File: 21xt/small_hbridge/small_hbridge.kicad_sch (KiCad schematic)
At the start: 3 parts, among them J1 Conn_01x03, J2 Conn_01x02, J3 Barrel_Jack

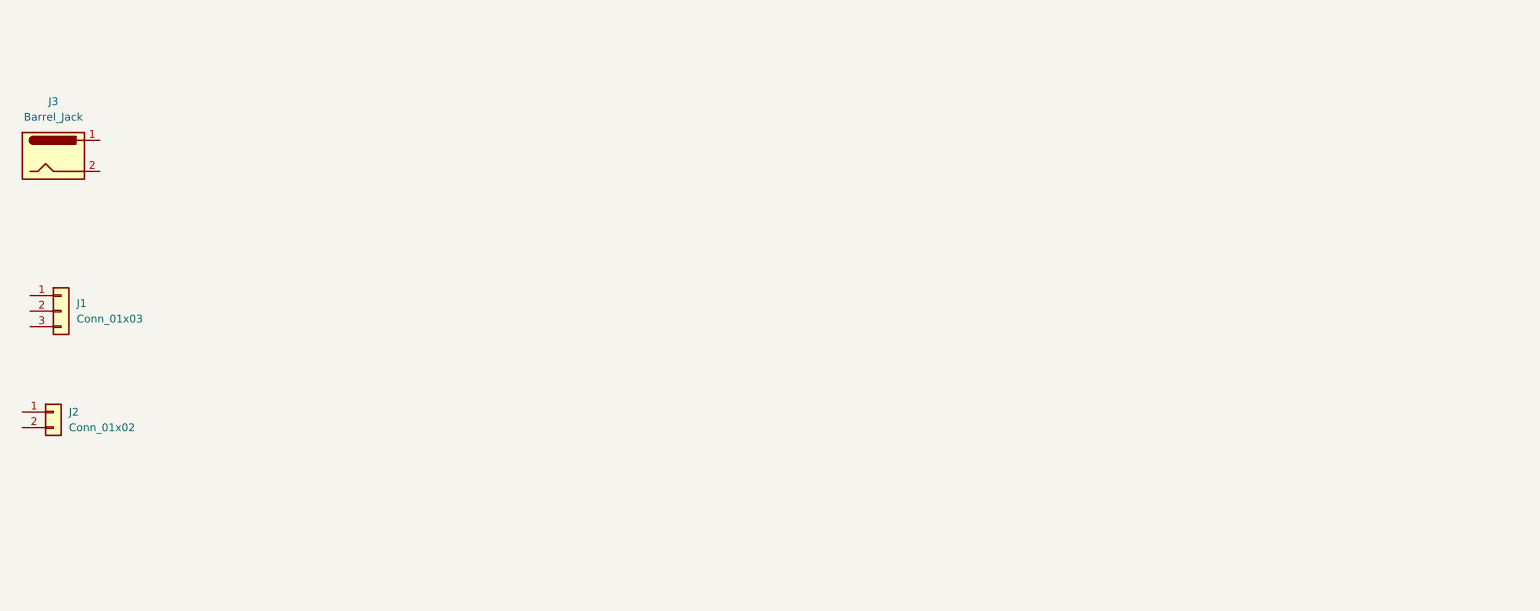
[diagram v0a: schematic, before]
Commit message: aaaaa
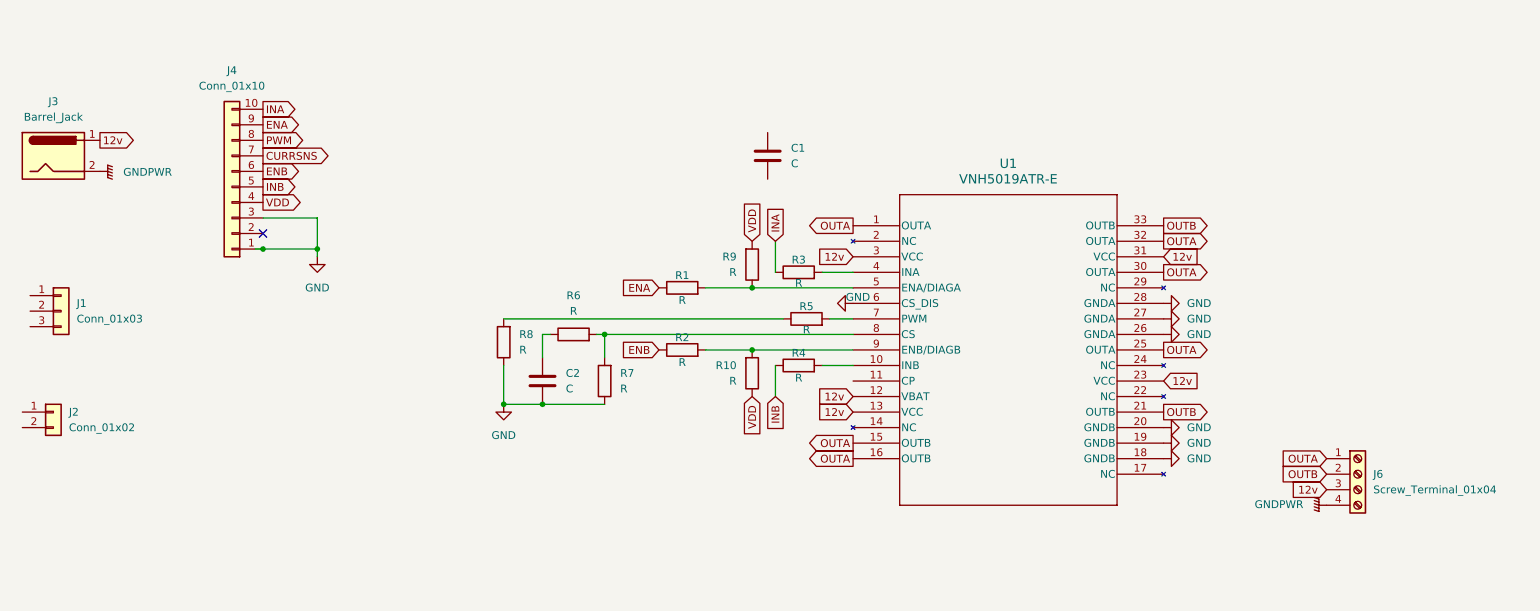
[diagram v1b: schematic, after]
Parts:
- added C1, C2: C, symbol Device:C
- added J4: Conn_01x10, symbol Connector_Generic:Conn_01x10
- added J6: Screw_Terminal_01x04, symbol Connector:Screw_Terminal_01x04
- added R1, R10, R2, R3, R4, R5, R6, R7, R8, R9: R, symbol Device:R
- added U1: VNH5019ATR-E, MultiPowerSO-30_STM, symbol dyno_inst_sym:VNH5019ATR-E
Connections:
- net 12v: now reaches J3.1
- net 12v: now also J6.3 (Pin_3), U1.12 (VBAT), U1.13 (VCC), U1.23 (VCC), U1.3 (VCC), U1.31 (VCC)
- net GNDPWR: now reaches J3.2
- net GNDPWR: now also J6.4 (Pin_4)
- new net: R5.1, R8.2
- new net: R5.2, U1.7 (PWM)
- new net: C2.1, R6.1
- new net: R3.2, U1.4 (INA)
- new net: R6.2, R7.2, U1.8 (CS)
- new net: R4.2, U1.10 (INB)
- new net: R1.2, R9.1, U1.5 (ENA/DIAGA)
- new net: R10.2, R2.2, U1.9 (ENB/DIAGB)
- new net CURRSNS: J4.7 (Pin_7)
- new net ENA: J4.9 (Pin_9), R1.1
- new net ENB: J4.6 (Pin_6), R2.1
- new net GND: C2.2, J4.1 (Pin_1), J4.3 (Pin_3), R7.1, R8.1, U1.18 (GNDB), U1.19 (GNDB), U1.20 (GNDB), U1.26 (GNDA), U1.27 (GNDA), U1.28 (GNDA), U1.6 (CS_DIS)
- new net INA: J4.10 (Pin_10), R3.1
- new net INB: J4.5 (Pin_5), R4.1
- new net OUTA: J6.1 (Pin_1), U1.1 (OUTA), U1.15 (OUTB), U1.16 (OUTB), U1.25 (OUTA), U1.30 (OUTA), U1.32 (OUTA)
- new net OUTB: J6.2 (Pin_2), U1.21 (OUTB), U1.33 (OUTB)
- new net PWM: J4.8 (Pin_8)
- new net VDD: J4.4 (Pin_4), R10.1, R9.2
- no-connect marks 0 -> 1

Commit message: ssss
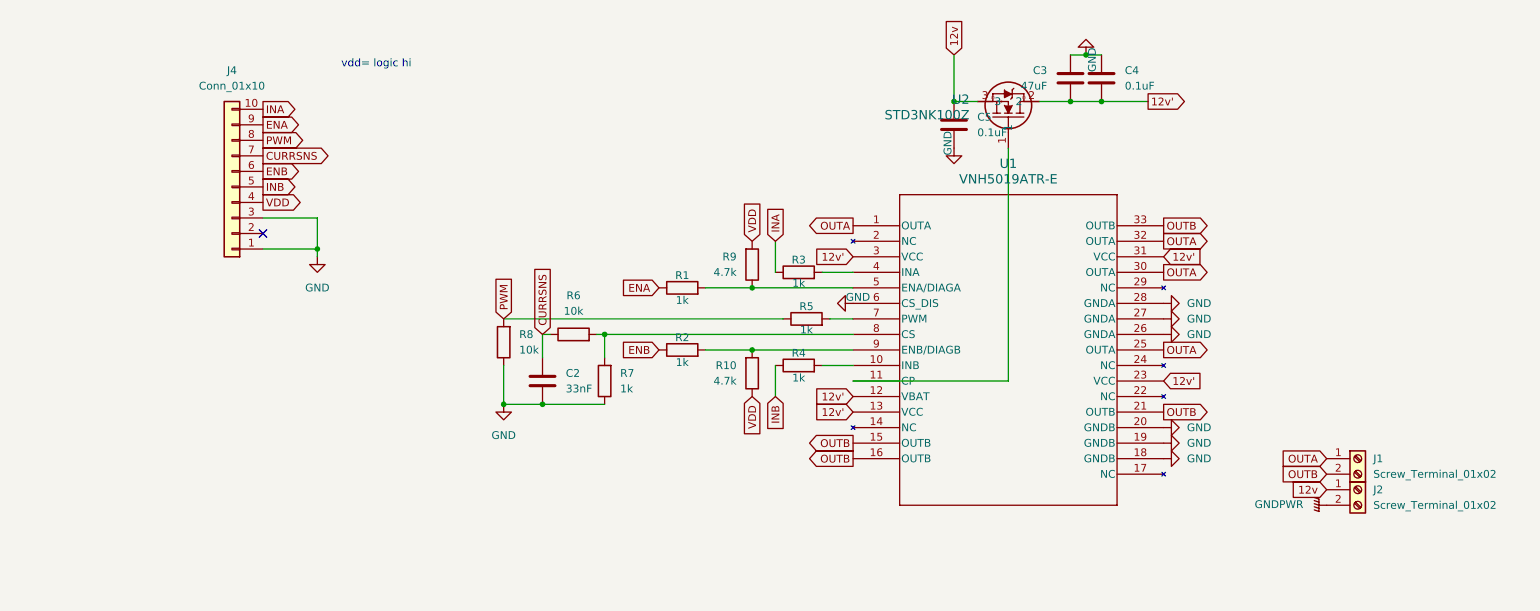
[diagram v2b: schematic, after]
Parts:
- removed C1: C, symbol Device:C
- removed J1: Conn_01x03, symbol Connector_Generic:Conn_01x03
- removed J2: Conn_01x02, symbol Connector_Generic:Conn_01x02
- removed J3: Barrel_Jack, symbol Connector:Barrel_Jack
- removed J6: Screw_Terminal_01x04, symbol Connector:Screw_Terminal_01x04
- added C3: 47uF, Capacitor_SMD:C_0603_1608Metric, symbol Device:C
- added C4, C5: 0.1uF, Capacitor_SMD:C_0603_1608Metric, symbol Device:C
- added J1, J2: Screw_Terminal_01x02, dynoinst_fp:CONN_4DB-P108-02_TEC, symbol Connector:Screw_Terminal_01x02
- added U2: STD3NK100Z, DPAK_STM, symbol dyno_inst_sym:STD3NK100Z
- C2: value C -> 33nF; footprint (none) -> Capacitor_SMD:C_0603_1608Metric
- J4: footprint (none) -> Connector_PinHeader_2.54mm:PinHeader_1x10_P2.54mm_Vertical
- R1, R2, R3, R4, R5, R7: value R -> 1k; footprint (none) -> Resistor_SMD:R_0603_1608Metric
- R10, R9: value R -> 4.7k; footprint (none) -> Resistor_SMD:R_0603_1608Metric
- R6, R8: value R -> 10k; footprint (none) -> Resistor_SMD:R_0603_1608Metric
- U1: footprint MultiPowerSO-30_STM -> dynoinst_fp:MultiPowerSO-30_STM
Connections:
- net 12v: now also C5.2, J2.1 (Pin_1), U2.3; no longer U1.12 (VBAT), U1.13 (VCC), U1.23 (VCC), U1.3 (VCC), U1.31 (VCC)
- net CURRSNS: now also C2.1, R6.1
- net GND: now also C3.1, C4.1, C5.1
- net GNDPWR: now also J2.2 (Pin_2)
- net OUTA: now also J1.1 (Pin_1); no longer U1.15 (OUTB), U1.16 (OUTB)
- net OUTB: now also U1.15 (OUTB), U1.16 (OUTB), J1.2 (Pin_2)
- net PWM: now also R5.1, R8.2
- net at U1.11 (CP): now also U2.1
- new net 12v': C3.2, C4.2, U1.12 (VBAT), U1.13 (VCC), U1.23 (VCC), U1.3 (VCC), U1.31 (VCC), U2.2
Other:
- note added: "vdd= logic hi"

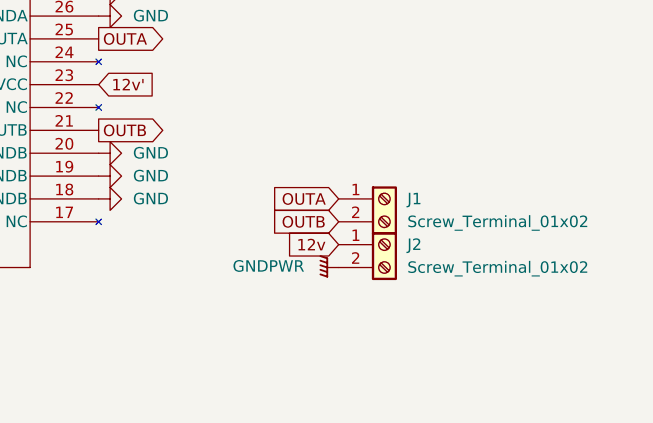
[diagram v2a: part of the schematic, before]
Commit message: aaaaa
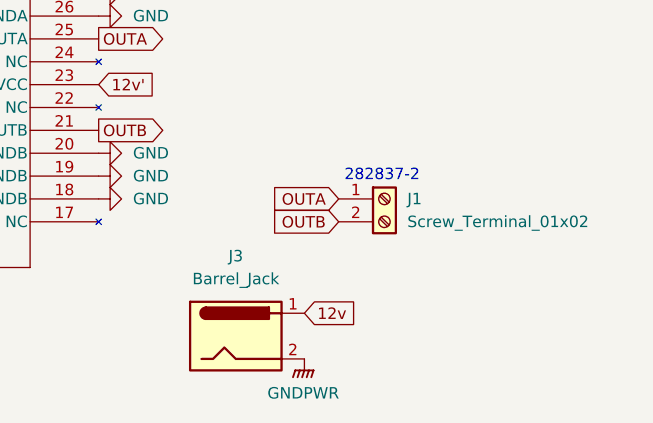
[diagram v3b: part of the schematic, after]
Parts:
- removed J2: Screw_Terminal_01x02, dynoinst_fp:CONN_4DB-P108-02_TEC, symbol Connector:Screw_Terminal_01x02
- added J3: Barrel_Jack, dynoinst_fp:CUI_PJ-037A, symbol Connector:Barrel_Jack
- J1: footprint dynoinst_fp:CONN_4DB-P108-02_TEC -> dynoinst_fp:282837-2_TYC
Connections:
- net 12v: now also J3.1
- net GNDPWR: now also J3.2
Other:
- note added: "282837-2"
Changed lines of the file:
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@@
+		)
+	)
+	(text "282837-2"
+		(exclude_from_sim no)
+		(at 271.526 81.28 0)
+		(effects
+			(font
+				(size 1.27 1.27)
+			)
 		)
 	)
@@
 		)
 	)
+	(global_label "12v"
+		(shape input)
+		(at 262.89 96.52 0)
+		(fields_autoplaced yes)
+		(effects
+			(font
+				(size 1.27 1.27)
+			)
+			(justify left)
+		)
+		(property "Intersheetrefs" "${INTERSHEET_REFS}"
+			(at 269.2618 96.52 0)
+			(effects
+				(font
+					(size 1.27 1.27)
+				)
+				(justify left)
+				(hide yes)
+			)
+		)
+	)
 	(global_label "CURRSNS"
 		(shape output)
@@
 		)
 	)
-	(global_label "12v"
-		(shape input)
-		(at 266.7 88.9 180)
-		(fields_autoplaced yes)
-		(effects
-			(font
-				(size 1.27 1.27)
-			)
-			(justify right)
-		)
-		(property "Intersheetrefs" "${INTERSHEET_REFS}"
-			(at 260.3282 88.9 0)
-			(effects
-				(font
-					(size 1.27 1.27)
-				)
-				(justify right)
-				(hide yes)
-			)
-		)
-	)
 	(global_label "OUTA"
 		(shape output)
@@
 	)
 	(symbol
-		(lib_id "power:GNDPWR")
-		(at 266.7 91.44 270)
-		(unit 1)
-		(exclude_from_sim no)
-		(in_bom yes)
-		(on_board yes)
-		(dnp no)
-		(fields_autoplaced yes)
-		(property "Reference" "#PWR011"
-			(at 261.62 91.44 0)
-			(effects
-				(font
-					(size 1.27 1.27)
-				)
-				(hide yes)
-			)
-		)
-		(property "Value" "GNDPWR"
-			(at 262.89 91.3129 90)
-			(effects
-				(font
-					(size 1.27 1.27)
-				)
-				(justify right)
-			)
-		)
-		(property "Footprint" ""
-			(at 265.43 91.44 0)
-			(effects
-				(font
-					(size 1.27 1.27)
-				)
-				(hide yes)
-			)
-		)
-		(property "Datasheet" ""
-			(at 265.43 91.44 0)
-			(effects
-				(font
-					(size 1.27 1.27)
-				)
-				(hide yes)
-			)
-		)
-		(property "Description" "Power symbol creates a global label with name \"GNDPWR\" , global ground"
-			(at 266.7 91.44 0)
-			(effects
-				(font
-					(size 1.27 1.27)
-				)
-				(hide yes)
-			)
-		)
-		(pin "1"
-		)
-		(instances
-			(project "small_hbridge"
-				(path "/316bab56-41f8-4598-8c04-8ef3331139a9"
-					(reference "#PWR011")
-					(unit 1)
-				)
-			)
-		)
-	)
-	(symbol
 		(lib_id "Device:R")
 		(at 181.61 60.96 90)
@@
 				(path "/316bab56-41f8-4598-8c04-8ef3331139a9"
 					(reference "R7")
+					(unit 1)
+				)
+			)
+		)
+	)
+	(symbol
+		(lib_id "Connector:Barrel_Jack")
+		(at 255.27 99.06 0)
+		(unit 1)
+		(exclude_from_sim no)
+		(in_bom yes)
+		(on_board yes)
+		(dnp no)
+		(fields_autoplaced yes)
+		(property "Reference" "J3"
+			(at 255.27 90.17 0)
+			(effects
+				(font
+					(size 1.27 1.27)
+				)
+			)
+		)
+		(property "Value" "Barrel_Jack"
+			(at 255.27 92.71 0)
+			(effects
+				(font
+					(size 1.27 1.27)
+				)
+			)
+		)
+		(property "Footprint" "dynoinst_fp:CUI_PJ-037A"
+			(at 256.54 100.076 0)
+			(effects
+				(font
+					(size 1.27 1.27)
+				)
+				(hide yes)
+			)
+		)
+		(property "Datasheet" "~"
+			(at 256.54 100.076 0)
+			(effects
+				(font
+					(size 1.27 1.27)
+				)
+				(hide yes)
+			)
+		)
+		(property "Description" "DC Barrel Jack"
+			(at 255.27 99.06 0)
+			(effects
+				(font
+					(size 1.27 1.27)
+				)
+				(hide yes)
+			)
+		)
+		(pin "2"
+		)
+		(pin "1"
+		)
+		(instances
+			(project "small_hbridge"
+				(path "/316bab56-41f8-4598-8c04-8ef3331139a9"
+					(reference "J3")
 					(unit 1)
 				)
@@
 	)
 	(symbol
-		(lib_id "Connector:Screw_Terminal_01x02")
-		(at 271.78 88.9 0)
-		(unit 1)
-		(exclude_from_sim no)
-		(in_bom yes)
-		(on_board yes)
-		(dnp no)
-		(fields_autoplaced yes)
-		(property "Reference" "J2"
-			(at 274.32 88.8999 0)
-			(effects
-				(font
-					(size 1.27 1.27)
-				)
-				(justify left)
-			)
-		)
-		(property "Value" "Screw_Terminal_01x02"
-			(at 274.32 91.4399 0)
-			(effects
-				(font
-					(size 1.27 1.27)
-				)
-				(justify left)
-			)
-		)
-		(property "Footprint" "dynoinst_fp:CONN_4DB-P108-02_TEC"
-			(at 271.78 88.9 0)
-			(effects
-				(font
-					(size 1.27 1.27)
-				)
-				(hide yes)
-			)
-		)
-		(property "Datasheet" "~"
-			(at 271.78 88.9 0)
-			(effects
-				(font
-					(size 1.27 1.27)
-				)
-				(hide yes)
-			)
-		)
-		(property "Description" "Generic screw terminal, single row, 01x02, script generated (kicad-library-utils/schlib/autogen/connector/)"
-			(at 271.78 88.9 0)
-			(effects
-				(font
-					(size 1.27 1.27)
-				)
-				(hide yes)
-			)
-		)
-		(pin "2"
-		)
-		(pin "1"
-		)
-		(instances
-			(project "small_hbridge"
-				(path "/316bab56-41f8-4598-8c04-8ef3331139a9"
-					(reference "J2")
-					(unit 1)
-				)
-			)
-		)
-	)
-	(symbol
 		(lib_id "Device:R")
 		(at 172.72 52.07 0)
@@
 	)
 	(symbol
+		(lib_id "power:GNDPWR")
+		(at 262.89 101.6 0)
+		(unit 1)
+		(exclude_from_sim no)
+		(in_bom yes)
+		(on_board yes)
+		(dnp no)
+		(fields_autoplaced yes)
+		(property "Reference" "#PWR03"
+			(at 262.89 106.68 0)
+			(effects
+				(font
+					(size 1.27 1.27)
+				)
+				(hide yes)
+			)
+		)
+		(property "Value" "GNDPWR"
+			(at 262.763 105.41 0)
+			(effects
+				(font
+					(size 1.27 1.27)
+				)
+			)
+		)
+		(property "Footprint" ""
+			(at 262.89 102.87 0)
+			(effects
+				(font
+					(size 1.27 1.27)
+				)
+				(hide yes)
+			)
+		)
+		(property "Datasheet" ""
+			(at 262.89 102.87 0)
+			(effects
+				(font
+					(size 1.27 1.27)
+				)
+				(hide yes)
+			)
+		)
+		(property "Description" "Power symbol creates a global label with name \"GNDPWR\" , global ground"
+			(at 262.89 101.6 0)
+			(effects
+				(font
+					(size 1.27 1.27)
+				)
+				(hide yes)
+			)
+		)
+		(pin "1"
+		)
+		(instances
+			(project "small_hbridge"
+				(path "/316bab56-41f8-4598-8c04-8ef3331139a9"
+					(reference "#PWR03")
+					(unit 1)
+				)
+			)
+		)
+	)
+	(symbol
 		(lib_id "Device:R")
 		(at 161.29 55.88 90)
@@
 			)
 		)
-		(property "Footprint" "dynoinst_fp:CONN_4DB-P108-02_TEC"
+		(property "Footprint" "dynoinst_fp:282837-2_TYC"
 			(at 271.78 83.82 0)
 			(effects
